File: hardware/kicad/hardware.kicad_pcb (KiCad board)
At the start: 2 copper layers, 36 x 36 mm, 16 parts, among them J1 Conn_01x02_Pin, J2 USB_C_Receptacle_USB2.0_14P, J3 Conn_Coaxial, J4 Micro_SD_Card, U1 STM32L412CBTx, U2 BQ24074RGT, U3 NCP163AFCT330T2G, U4 MAX-M10S

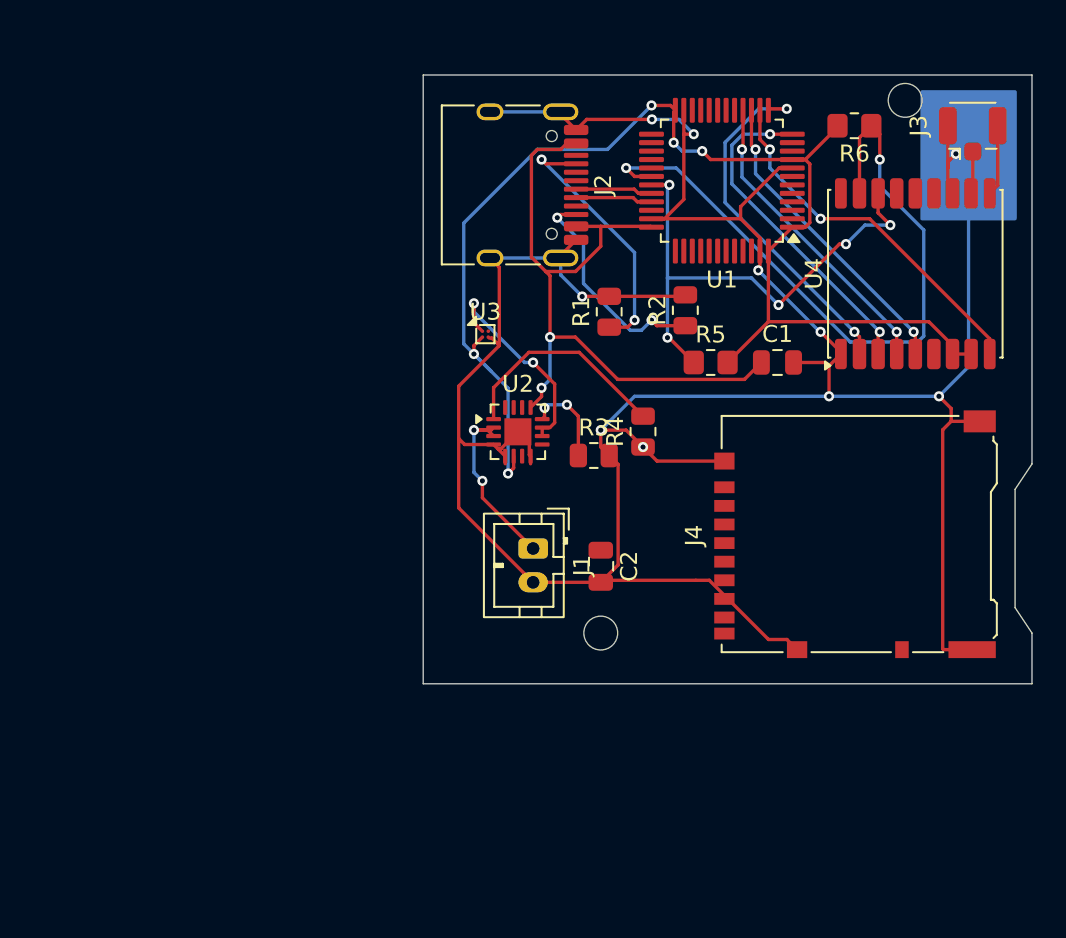
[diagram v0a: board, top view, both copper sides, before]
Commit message: reroute main pcb
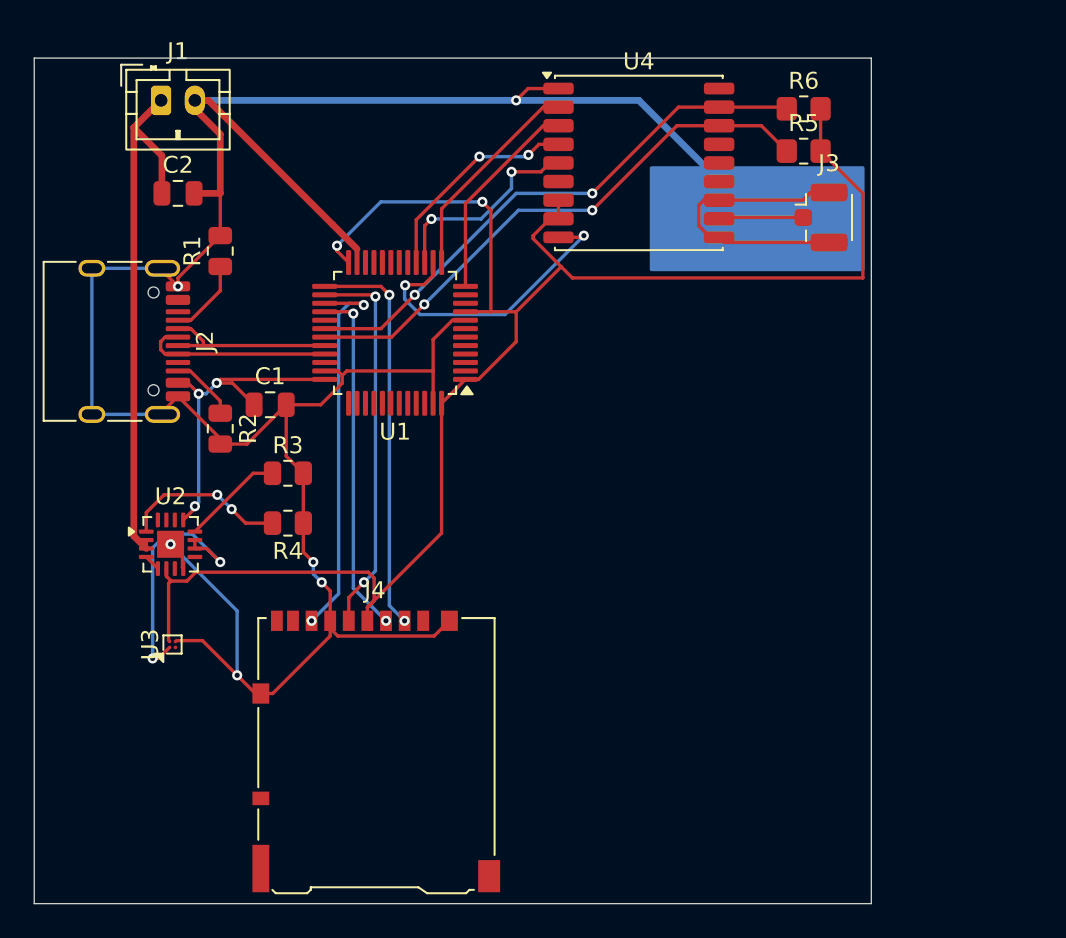
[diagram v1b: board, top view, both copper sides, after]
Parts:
- moved J1 34.4 mm to (109.5, 84.0), turned to 0 degrees
- moved C2 33.3 mm to (110.5, 89.5), turned to 0 degrees
- moved J4 31.1 mm to (122.2, 122.5), turned to 0 degrees
- moved C1 30.1 mm to (116.0, 102.0)
- moved R2 28.4 mm to (113.0, 103.4), turned to -90 degrees
- moved U3 26.1 mm to (110.2, 116.2), turned to 90 degrees
- moved J2 25.3 mm to (106.5, 98.2)
- moved R1 23.3 mm to (113.0, 92.9)
- moved R4 21.7 mm to (117.0, 109.0), turned to 180 degrees
- moved U2 21.6 mm to (110.1, 110.2)
- moved U1 21.3 mm to (123.3, 97.8)
- moved R3 18.1 mm to (117.0, 106.0)
- moved U4 17.6 mm to (137.8, 87.7), turned to 0 degrees
- moved R5 13.7 mm to (147.5, 87.0)
- moved J3 10.1 mm to (149.0, 90.9), turned to 0 degrees
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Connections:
- J4 pad 2: unconnected-(J4-DAT3/CD-Pad2) -> Net-(J4-DAT3/CD)
- J4 pad 3: unconnected-(J4-CMD-Pad3) -> Net-(J4-CMD)
- J4 pad 5: unconnected-(J4-CLK-Pad5) -> Net-(J4-CLK)
- J4 pad 7: unconnected-(J4-DAT0-Pad7) -> Net-(J4-DAT0)
- U1 pad 25: unconnected-(U1-PB12-Pad25) -> Net-(J4-DAT3/CD)
- U1 pad 26: unconnected-(U1-PB13-Pad26) -> Net-(J4-CLK)
- U1 pad 27: unconnected-(U1-PB14-Pad27) -> Net-(J4-DAT0)
- U1 pad 28: unconnected-(U1-PB15-Pad28) -> Net-(J4-CMD)
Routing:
- net +3.3V: track 75.7 -> 100.2 mm, vias 5 -> 2
- net Net-(J4-DAT3/CD): track 0.00 -> 23.7 mm, vias 0 -> 2
- net Net-(J4-DAT0): track 0.00 -> 22.9 mm, vias 0 -> 2
- net Net-(J4-CLK): track 0.00 -> 22.9 mm, vias 0 -> 2
- net Net-(U1-VDDUSB): track 42.3 -> 19.9 mm, vias 2 -> 3
- net Net-(J1-Pin_1): track 11.0 -> 32.5 mm, vias 2 -> 0
- net Net-(J4-CMD): track 0.00 -> 20.7 mm, vias 0 -> 2
- net GND: track 191.9 -> 176.9 mm, vias 10 -> 6
- net Net-(J2-CC1): track 15.6 -> 4.65 mm, vias 2 -> 0
- net Net-(J2-CC2): track 13.3 -> 3.96 mm, vias 2 -> 0
- net Net-(U1-PA9): track 41.7 -> 32.8 mm
- net Net-(U1-PA3): track 21.4 -> 12.6 mm, vias 2 -> 0
- net Net-(U1-PA2): track 19.9 -> 12.3 mm, vias 2 -> 0
- net Net-(U1-PA12): track 4.56 -> 11.4 mm
- net Net-(U1-PA5): track 18.4 -> 12.2 mm
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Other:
- board size 36 x 36 mm -> 49.5 x 50 mm
